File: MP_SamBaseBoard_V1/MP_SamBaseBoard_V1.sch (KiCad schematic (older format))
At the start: 142 parts, among them J1 MA_CONN, J10 P1_CONN, J11 I2C_CONN, J12 I2C_CONN, J13 SAM_SWD, J14 WS2812_EXT, J15 PWR_JACK, J16 USB_B_Micro, J17 BATT_CONN, J2 MB_CONN, J3 Adafruit_Feather_CONN, J4 LOAD_CONN, J5 SPEAKER, J7 SERVO_CONN, J8 P3_CONN, J9 P2_CONN, Q1 DMP3098L, Q2 ALS-PT19-315C/L177/TR8, Q3 BSS138-7-F, SW1 RESET, SW2 3v3_PWR_SW, SW3 SW1, SW4 SW2, U1 ESP32-WROOM-32, U10 KXTJ3-1057, U11 IRFHM3911PbF, U12 IRFHM9331PbF, U13 SST25VF016B-50-4C-S2AF, U14 IRFHM9331PbF, U2 ATSAMD51J19A-A, U3 74LVC1G125, U4 TPS62135, U5 PAM8301, U6 BQ24075, U7 DRV8833RTY, U8 Sensirion_SHT3x, U9 LD39200PU33R, Y1 Crystal

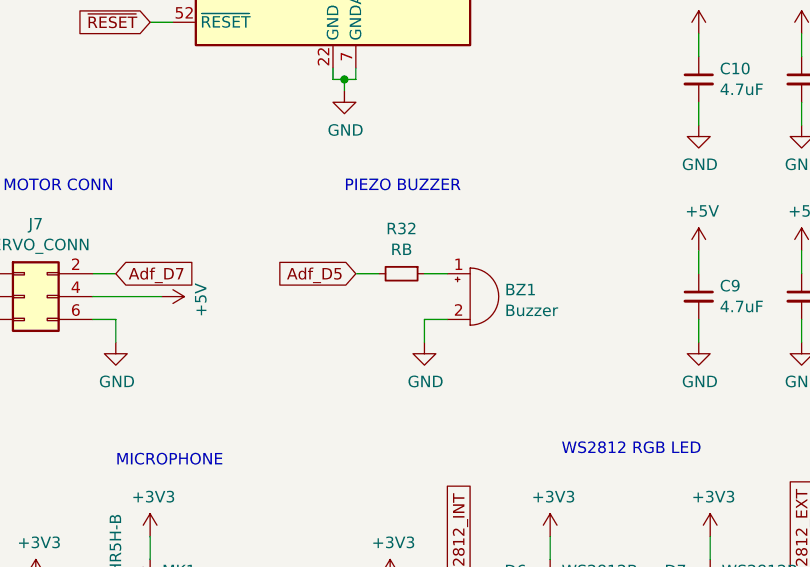
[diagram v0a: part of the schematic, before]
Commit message: Update design
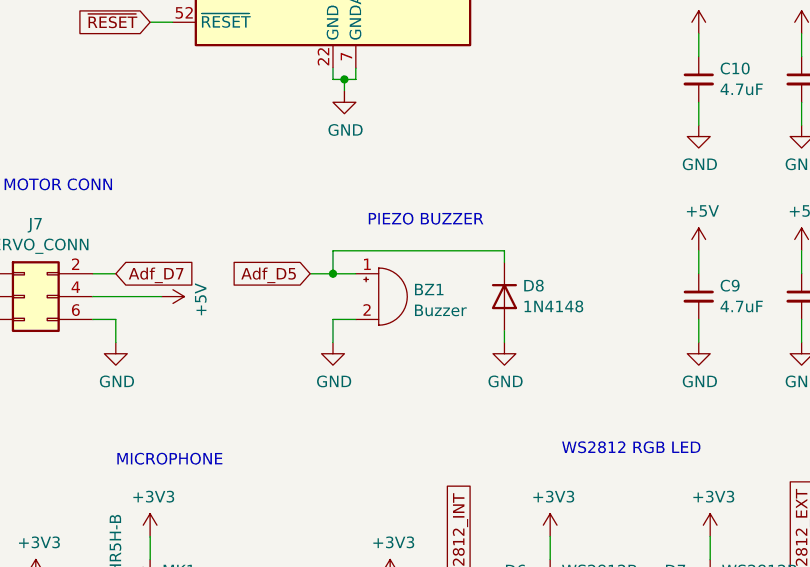
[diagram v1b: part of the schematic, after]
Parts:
- removed R32: RB, Resistor_SMD:R_0603_1608Metric, symbol Device:R_Small
- added D8: 1N4148, Diode_SMD:D_SOD-123, symbol Diode:1N4148
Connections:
- net Adf_D5: now also BZ1.1 (-), D8.1 (K)
- net GND: now also D8.2 (A)
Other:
- moved on the sheet: BZ1
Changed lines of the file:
@@
 EESchema Schematic File Version 4
-LIBS:MP_SamBaseBoard_V1-cache
-EELAYER 26 0
+EELAYER 30 0
 EELAYER END
 $Descr A3 16535 11693
@@
 Text Notes 12200 10950 0    59   ~ 0
 Maker Playground SAMD Cortex M4F + ESP32 Base Board
-Text GLabel 7550 6550 0    50   Input ~ 0
+Text GLabel 7350 6550 0    50   Input ~ 0
 Adf_D5
 $Comp
 L Device:Buzzer BZ1
 U 1 1 5ED7BCD8
-P 8050 6650
-F 0 "BZ1" H 8202 6679 50  0000 L CNN
-F 1 "Buzzer" H 8202 6588 50  0000 L CNN
-F 2 "Buzzer_Beeper:MagneticBuzzer_Kobitone_254-EMB84Q-RO" V 8025 6750 50  0001 C CNN
-F 3 "~" V 8025 6750 50  0001 C CNN
-	1    8050 6650
+P 7650 6650
+F 0 "BZ1" H 7802 6679 50  0000 L CNN
+F 1 "Buzzer" H 7802 6588 50  0000 L CNN
+F 2 "Buzzer_Beeper:MagneticBuzzer_Kobitone_254-EMB84Q-RO" V 7625 6750 50  0001 C CNN
+F 3 "~" V 7625 6750 50  0001 C CNN
+	1    7650 6650
 	1    0    0    -1
 $EndComp
 $Comp
-L Device:R_Small R32
-U 1 1 5ED7E16B
-P 7750 6550
-F 0 "R32" V 7554 6550 50  0000 C CNN
-F 1 "RB" V 7645 6550 50  0000 C CNN
-F 2 "Resistor_SMD:R_0603_1608Metric" H 7750 6550 50  0001 C CNN
-F 3 "~" H 7750 6550 50  0001 C CNN
-	1    7750 6550
-	0    1    1    0
-$EndComp
-Wire Wire Line
-	7550 6550 7650 6550
-Wire Wire Line
-	7850 6550 7950 6550
-$Comp
 L power:GND #PWR0232
 U 1 1 5EE434AE
-P 7850 6850
-F 0 "#PWR0232" H 7850 6600 50  0001 C CNN
-F 1 "GND" H 7855 6677 50  0000 C CNN
-F 2 "" H 7850 6850 50  0001 C CNN
-F 3 "" H 7850 6850 50  0001 C CNN
-	1    7850 6850
+P 7450 6850
+F 0 "#PWR0232" H 7450 6600 50  0001 C CNN
+F 1 "GND" H 7455 6677 50  0000 C CNN
+F 2 "" H 7450 6850 50  0001 C CNN
+F 3 "" H 7450 6850 50  0001 C CNN
+	1    7450 6850
 	1    0    0    -1
 $EndComp
 Wire Wire Line
-	7850 6850 7850 6750
+	7450 6850 7450 6750
 Wire Wire Line
-	7850 6750 7950 6750
+	7450 6750 7550 6750
 $Comp
 L Connector:USB_B_Micro J16
@@
 	0    1    1    0
 $EndComp
-Text Notes 7500 6200 0    50   ~ 0
+Text Notes 7600 6350 0    50   ~ 0
 PIEZO BUZZER
 Text GLabel 3700 5650 2    50   Input ~ 0
@@
 	9750 9150 9850 9150
 $Comp
-L power:+3V3 #PWR?
+L power:+3V3 #PWR0251
 U 1 1 5F0262F3
 P 9500 10250
-F 0 "#PWR?" H 9500 10100 50  0001 C CNN
+F 0 "#PWR0251" H 9500 10100 50  0001 C CNN
 F 1 "+3V3" V 9515 10378 50  0000 L CNN
 F 2 "" H 9500 10250 50  0001 C CNN
@@
 $EndComp
 $Comp
-L power:+3V3 #PWR?
+L power:+3V3 #PWR0252
 U 1 1 5F02665C
 P 10300 10250
-F 0 "#PWR?" H 10300 10100 50  0001 C CNN
+F 0 "#PWR0252" H 10300 10100 50  0001 C CNN
 F 1 "+3V3" V 10315 10378 50  0000 L CNN
 F 2 "" H 10300 10250 50  0001 C CNN
@@
 	1    0    0    -1
 $EndComp
+$Comp
+L Diode:1N4148 D8
+U 1 1 5F1B38A1
+P 8200 6650
+F 0 "D8" V 8154 6730 50  0000 L CNN
+F 1 "1N4148" V 8245 6730 50  0000 L CNN
+F 2 "Diode_SMD:D_SOD-123" H 8200 6475 50  0001 C CNN
+F 3 "https://assets.nexperia.com/documents/data-sheet/1N4148_1N4448.pdf" H 8200 6650 50  0001 C CNN
+	1    8200 6650
+	0    1    1    0
+$EndComp
+Wire Wire Line
+	7350 6550 7450 6550
+Wire Wire Line
+	7450 6550 7450 6450
+Wire Wire Line
+	7450 6450 8200 6450
+Wire Wire Line
+	8200 6450 8200 6500
+Connection ~ 7450 6550
+Wire Wire Line
+	7450 6550 7550 6550
+$Comp
+L power:GND #PWR0253
+U 1 1 5F455707
+P 8200 6850
+F 0 "#PWR0253" H 8200 6600 50  0001 C CNN
+F 1 "GND" H 8205 6677 50  0000 C CNN
+F 2 "" H 8200 6850 50  0001 C CNN
+F 3 "" H 8200 6850 50  0001 C CNN
+	1    8200 6850
+	1    0    0    -1
+$EndComp
+Wire Wire Line
+	8200 6800 8200 6850
 $EndSCHEMATC

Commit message: Update design
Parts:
- D8: footprint Diode_SMD:D_SOD-123 -> Diode_SMD:D_SOD-323
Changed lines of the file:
@@
 F 0 "D8" V 8154 6730 50  0000 L CNN
 F 1 "1N4148" V 8245 6730 50  0000 L CNN
-F 2 "Diode_SMD:D_SOD-123" H 8200 6475 50  0001 C CNN
+F 2 "Diode_SMD:D_SOD-323" H 8200 6475 50  0001 C CNN
 F 3 "https://assets.nexperia.com/documents/data-sheet/1N4148_1N4448.pdf" H 8200 6650 50  0001 C CNN
 	1    8200 6650
